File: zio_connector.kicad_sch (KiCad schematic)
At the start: 4 parts, among them CN10 Conn_02x17_Odd_Even, CN7 Conn_02x10_Odd_Even, CN8 Conn_02x08_Odd_Even, CN9 Conn_02x15_Odd_Even

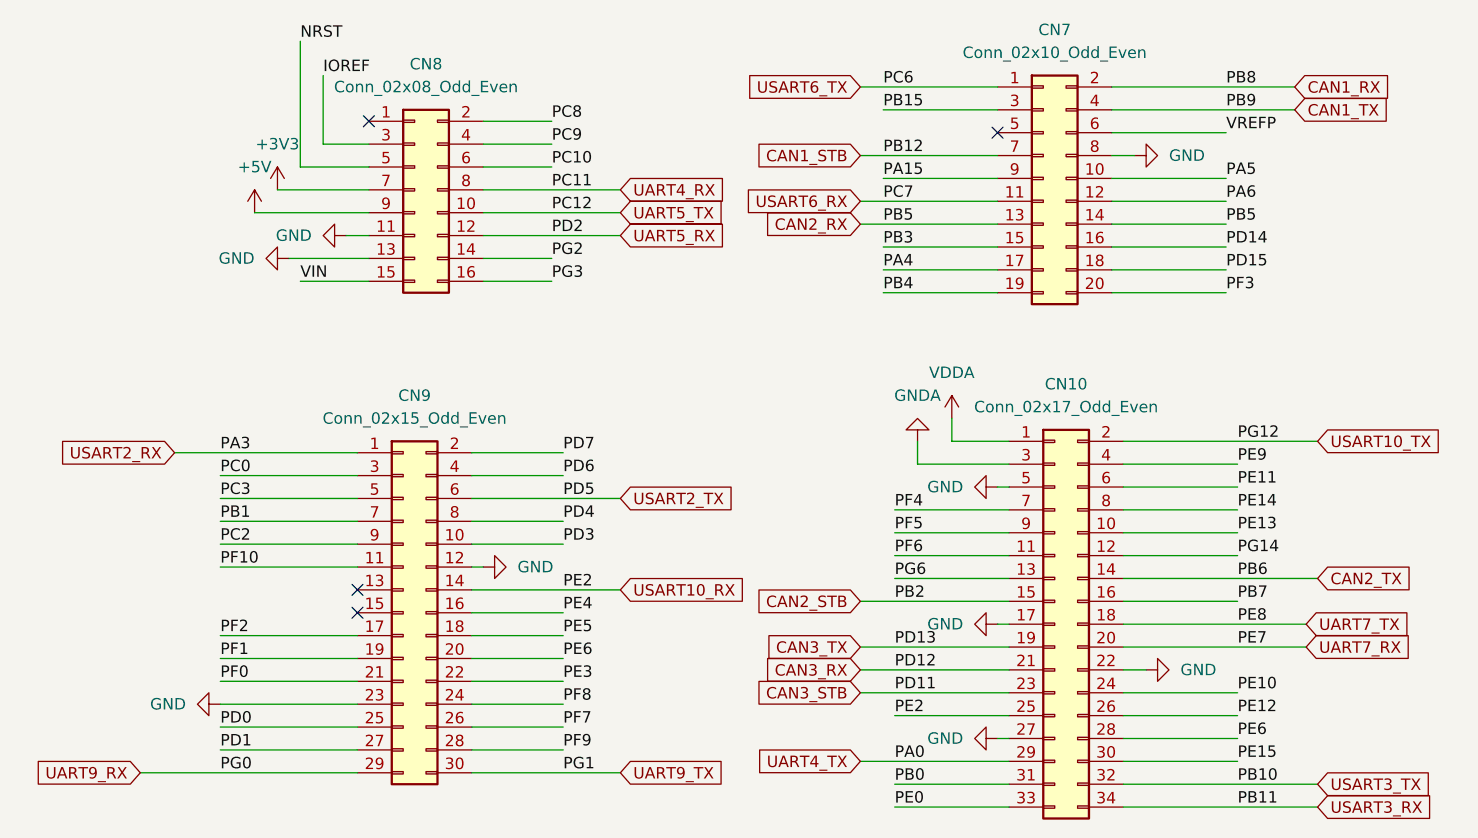
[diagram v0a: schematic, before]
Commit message: uarts routed
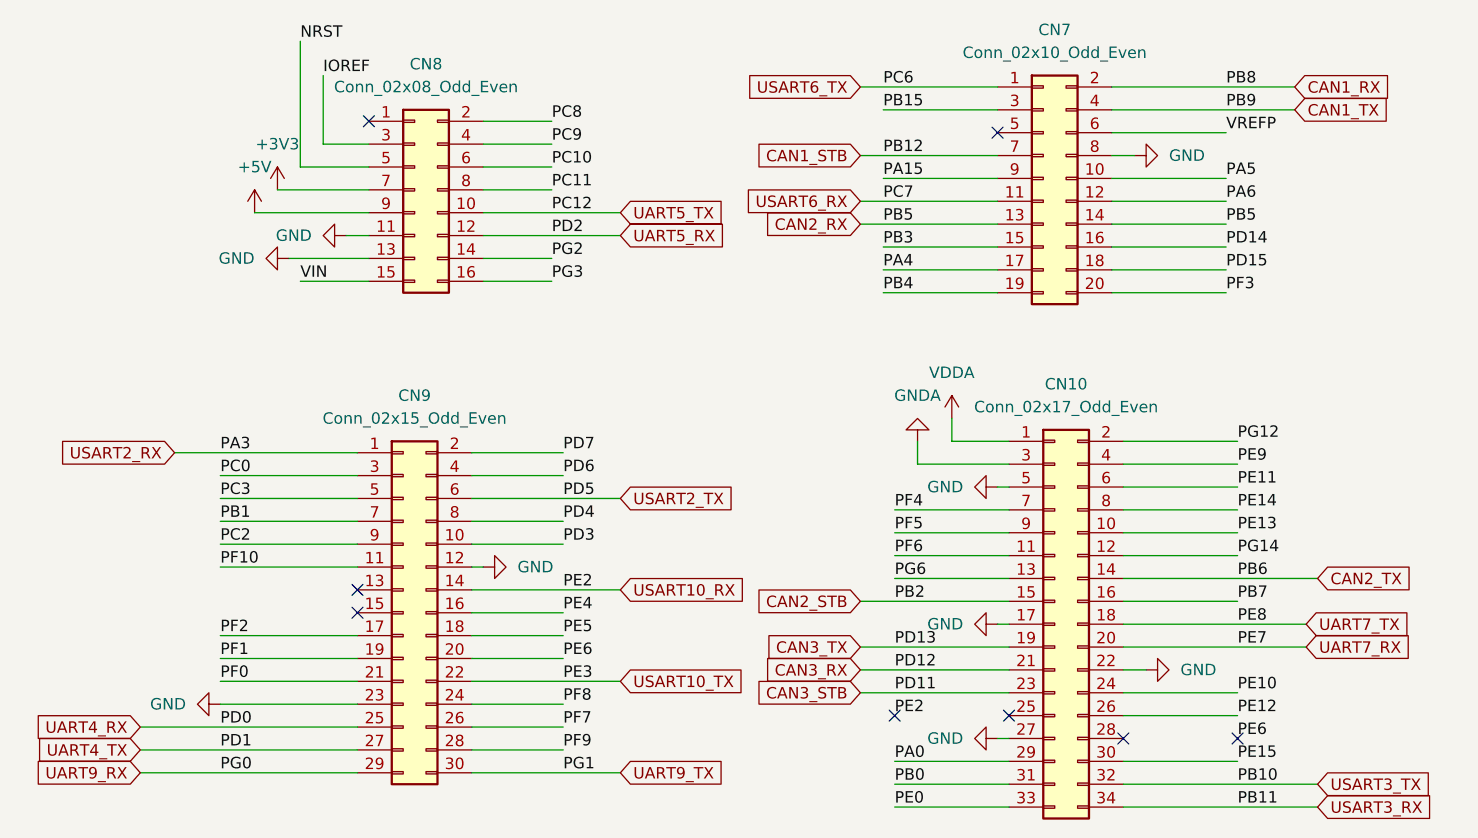
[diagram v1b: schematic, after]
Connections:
- net PD0 is gone; now on net UART4_RX: CN9.25 (Pin_25)
- net PD1 is gone; now on net UART4_TX: CN9.27 (Pin_27)
- net PE3 is gone; now on net USART10_TX: CN9.22 (Pin_22)
- net PE6: no longer CN10.28 (Pin_28)
- net UART4_RX: no longer CN8.8 (Pin_8)
- net UART4_TX: no longer CN10.29 (Pin_29)
- net USART10_RX: no longer CN10.25 (Pin_25)
- net USART10_TX: no longer CN10.2 (Pin_2)
- new net PA0: CN10.29 (Pin_29)
- new net PC11: CN8.8 (Pin_8)
- new net PG12: CN10.2 (Pin_2)
- no-connect marks 4 -> 8
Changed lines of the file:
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@@
 	(paper "A4")
 	(no_connect
+		(at 133.35 95.25)
+	)
+	(no_connect
 		(at 132.08 30.48)
 	)
@@
 	)
 	(no_connect
+		(at 146.05 97.79)
+	)
+	(no_connect
 		(at 60.96 81.28)
 	)
@@
 		(at 60.96 83.82)
 	)
+	(no_connect
+		(at 120.65 95.25)
+	)
+	(no_connect
+		(at 158.75 97.79)
+	)
 	(wire
 		(pts
@@
 	(wire
 		(pts
+			(xy 120.65 100.33) (xy 133.35 100.33)
+		)
+		(stroke
+			(width 0)
+			(type default)
+		)
+	)
+	(wire
+		(pts
 			(xy 119.38 35.56) (xy 132.08 35.56)
 		)
@@
 	(wire
 		(pts
-			(xy 74.93 36.83) (xy 90.17 36.83)
-		)
-		(stroke
-			(width 0)
-			(type default)
-		)
-	)
-	(wire
-		(pts
 			(xy 116.84 33.02) (xy 132.08 33.02)
 		)
@@
 	(wire
 		(pts
-			(xy 45.72 99.06) (xy 60.96 99.06)
-		)
-		(stroke
-			(width 0)
-			(type default)
-		)
-	)
-	(wire
-		(pts
 			(xy 144.78 27.94) (xy 165.1 27.94)
 		)
@@
 	(wire
 		(pts
+			(xy 74.93 36.83) (xy 82.55 36.83)
+		)
+		(stroke
+			(width 0)
+			(type default)
+		)
+	)
+	(wire
+		(pts
 			(xy 144.78 45.72) (xy 157.48 45.72)
 		)
@@
 	(wire
 		(pts
-			(xy 146.05 97.79) (xy 158.75 97.79)
-		)
-		(stroke
-			(width 0)
-			(type default)
-		)
-	)
-	(wire
-		(pts
 			(xy 73.66 76.2) (xy 83.82 76.2)
 		)
@@
 	(wire
 		(pts
-			(xy 146.05 64.77) (xy 167.64 64.77)
-		)
-		(stroke
-			(width 0)
-			(type default)
-		)
-	)
-	(wire
-		(pts
 			(xy 116.84 90.17) (xy 133.35 90.17)
 		)
@@
 	(wire
 		(pts
-			(xy 45.72 96.52) (xy 60.96 96.52)
-		)
-		(stroke
-			(width 0)
-			(type default)
-		)
-	)
-	(wire
-		(pts
 			(xy 53.34 44.45) (xy 62.23 44.45)
 		)
@@
 	(wire
 		(pts
+			(xy 146.05 64.77) (xy 158.75 64.77)
+		)
+		(stroke
+			(width 0)
+			(type default)
+		)
+	)
+	(wire
+		(pts
 			(xy 116.84 82.55) (xy 133.35 82.55)
 		)
@@
 	(wire
 		(pts
-			(xy 116.84 100.33) (xy 133.35 100.33)
-		)
-		(stroke
-			(width 0)
-			(type default)
-		)
-	)
-	(wire
-		(pts
 			(xy 49.53 39.37) (xy 62.23 39.37)
 		)
@@
 	(wire
 		(pts
-			(xy 73.66 91.44) (xy 83.82 91.44)
+			(xy 36.83 96.52) (xy 60.96 96.52)
+		)
+		(stroke
+			(width 0)
+			(type default)
+		)
+	)
+	(wire
+		(pts
+			(xy 73.66 91.44) (xy 90.17 91.44)
 		)
 		(stroke
@@
 	(wire
 		(pts
-			(xy 120.65 95.25) (xy 133.35 95.25)
-		)
-		(stroke
-			(width 0)
-			(type default)
-		)
-	)
-	(wire
-		(pts
 			(xy 146.05 100.33) (xy 158.75 100.33)
 		)
@@
 		(pts
 			(xy 116.84 87.63) (xy 133.35 87.63)
+		)
+		(stroke
+			(width 0)
+			(type default)
+		)
+	)
+	(wire
+		(pts
+			(xy 36.83 99.06) (xy 60.96 99.06)
 		)
 		(stroke
@@
 	(global_label "UART4_RX"
 		(shape input)
-		(at 90.17 36.83 0)
-		(fields_autoplaced yes)
-		(effects
-			(font
-				(size 1.27 1.27)
-			)
-			(justify left)
+		(at 36.83 96.52 180)
+		(fields_autoplaced yes)
+		(effects
+			(font
+				(size 1.27 1.27)
+			)
+			(justify right)
 		)
 		(property "Intersheetrefs" "${INTERSHEET_REFS}"
-			(at 102.4685 36.83 0)
+			(at 24.5315 96.52 0)
 			(effects
 				(font
 					(size 1.27 1.27)
 				)
-				(justify left)
+				(justify right)
 				(hide yes)
 			)
@@
 	(global_label "USART10_TX"
 		(shape input)
-		(at 167.64 64.77 0)
+		(at 90.17 91.44 0)
 		(fields_autoplaced yes)
 		(effects
@@
 		)
 		(property "Intersheetrefs" "${INTERSHEET_REFS}"
-			(at 182.0551 64.77 0)
+			(at 104.5851 91.44 0)
 			(effects
 				(font
@@
 	(global_label "UART4_TX"
 		(shape input)
-		(at 116.84 100.33 180)
+		(at 36.83 99.06 180)
 		(fields_autoplaced yes)
 		(effects
@@
 		)
 		(property "Intersheetrefs" "${INTERSHEET_REFS}"
-			(at 104.8439 100.33 0)
+			(at 24.8339 99.06 0)
 			(effects
 				(font
